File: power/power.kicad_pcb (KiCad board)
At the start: 2 copper layers, 60 x 60 mm, 22 parts, among them J1 XT30, J2 JST Terminal, U1 AP63200WU, U2 AP63200WU

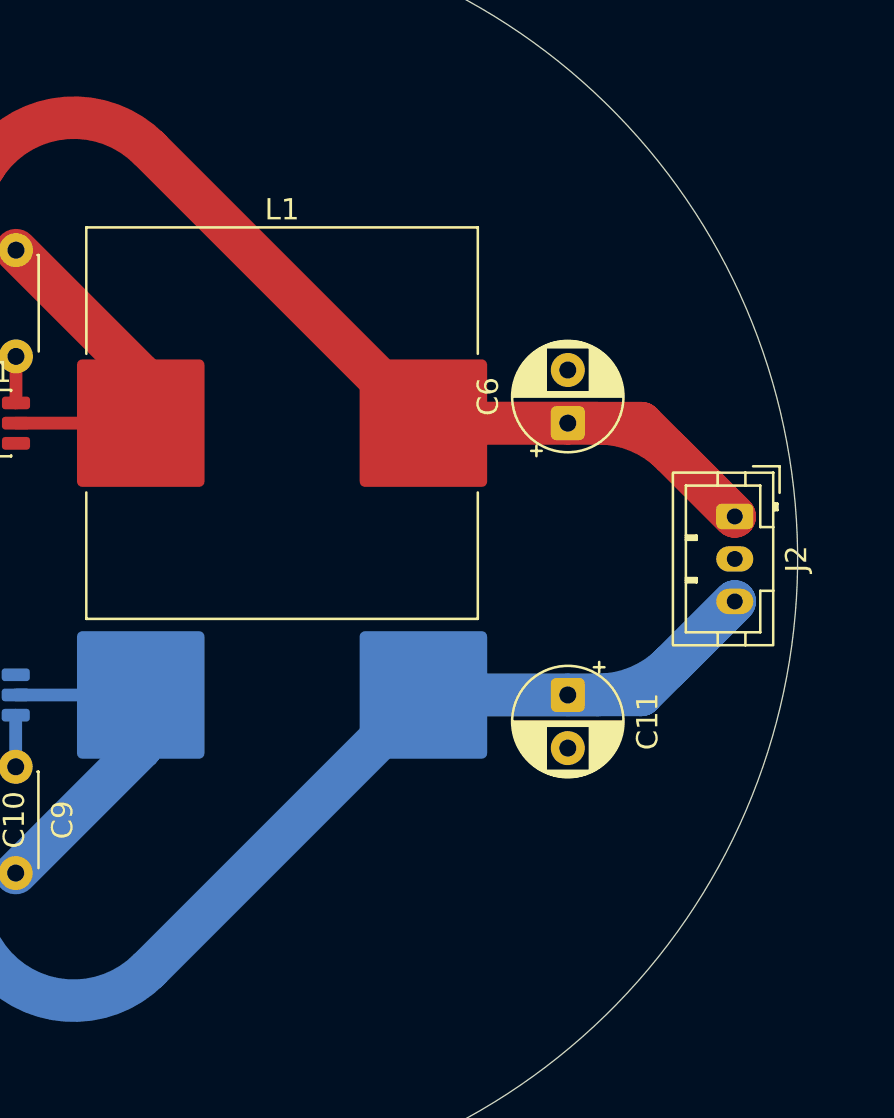
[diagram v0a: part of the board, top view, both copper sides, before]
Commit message: refresh
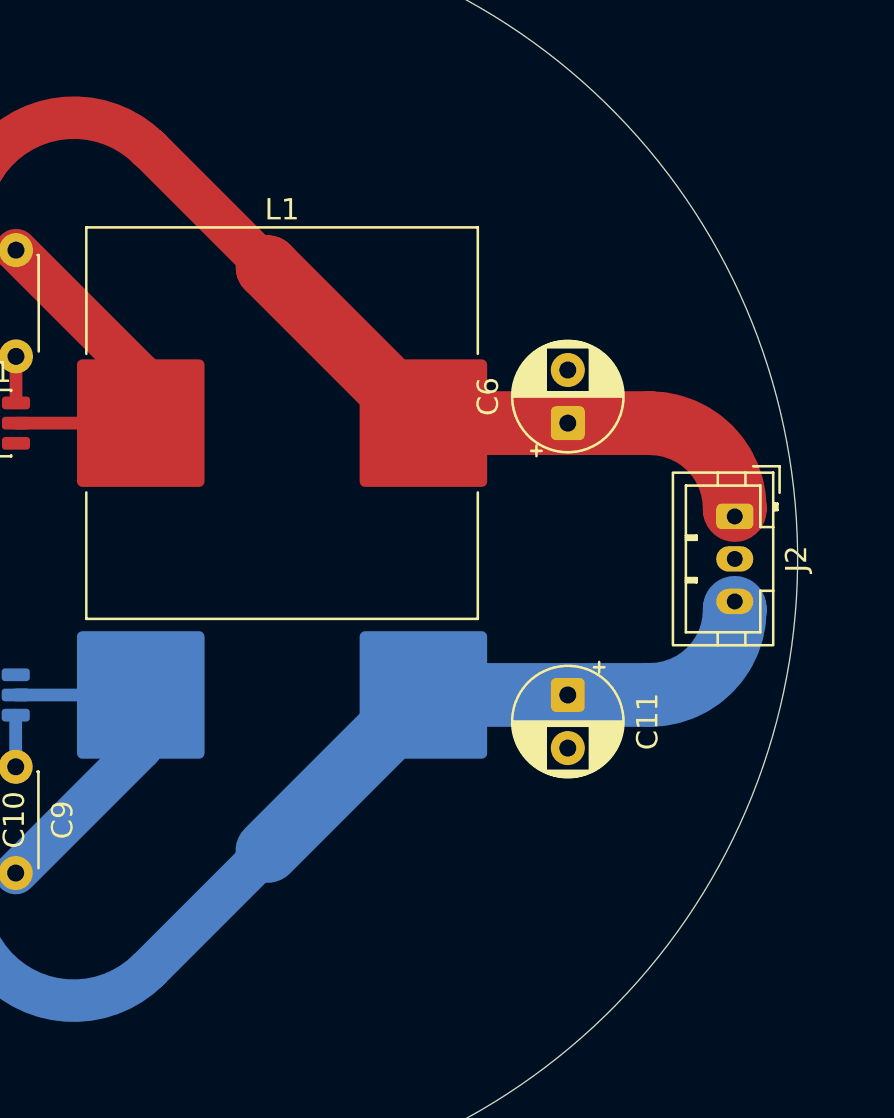
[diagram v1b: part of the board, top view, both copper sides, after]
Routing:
- net Net-(J2-Pin_3): track 88.8 -> 73.0 mm
- net Net-(J2-Pin_1): track 87.9 -> 72.0 mm
